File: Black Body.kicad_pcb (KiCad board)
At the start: 2 copper layers, 55 x 53.8 mm, 36 parts, among them IC2 MCP96L00T-E_MX, J1 53307-2471, J3 Conn_01x04, J4 MX150_02x08_RightAngle

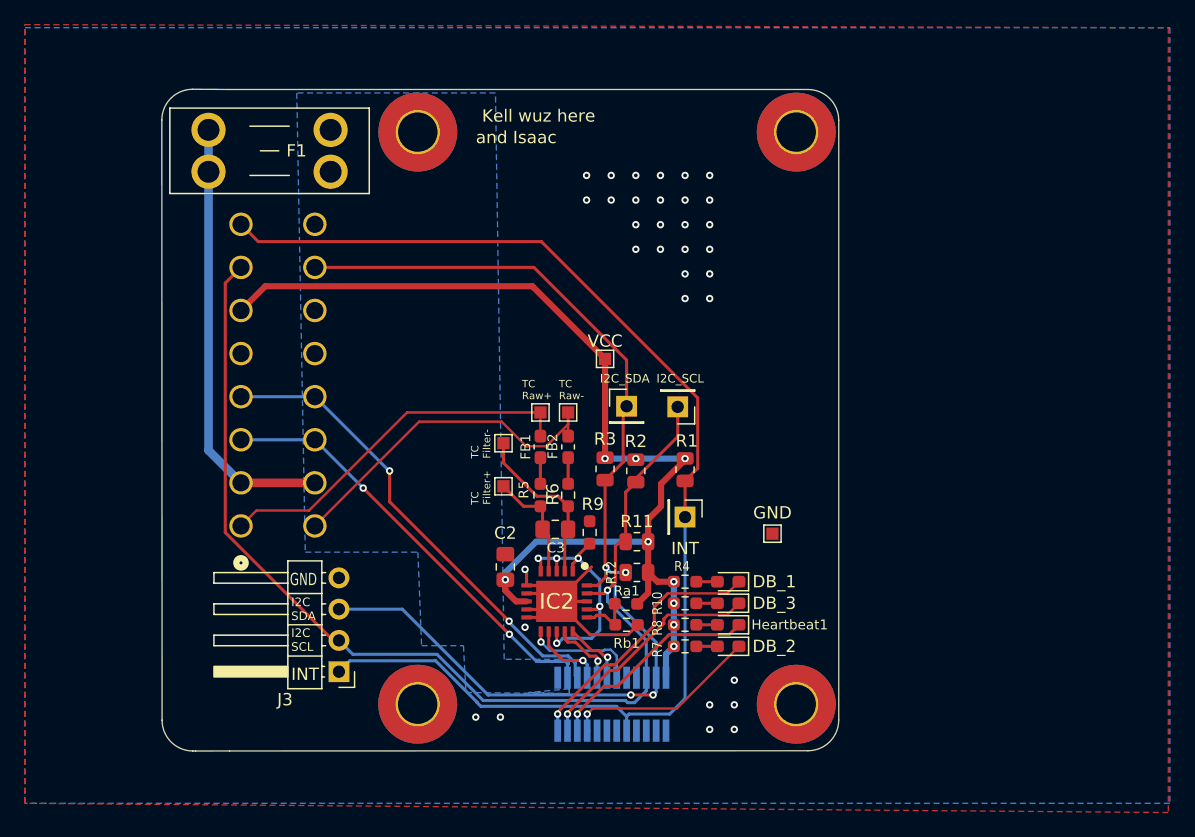
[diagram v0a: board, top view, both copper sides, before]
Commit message: better file system
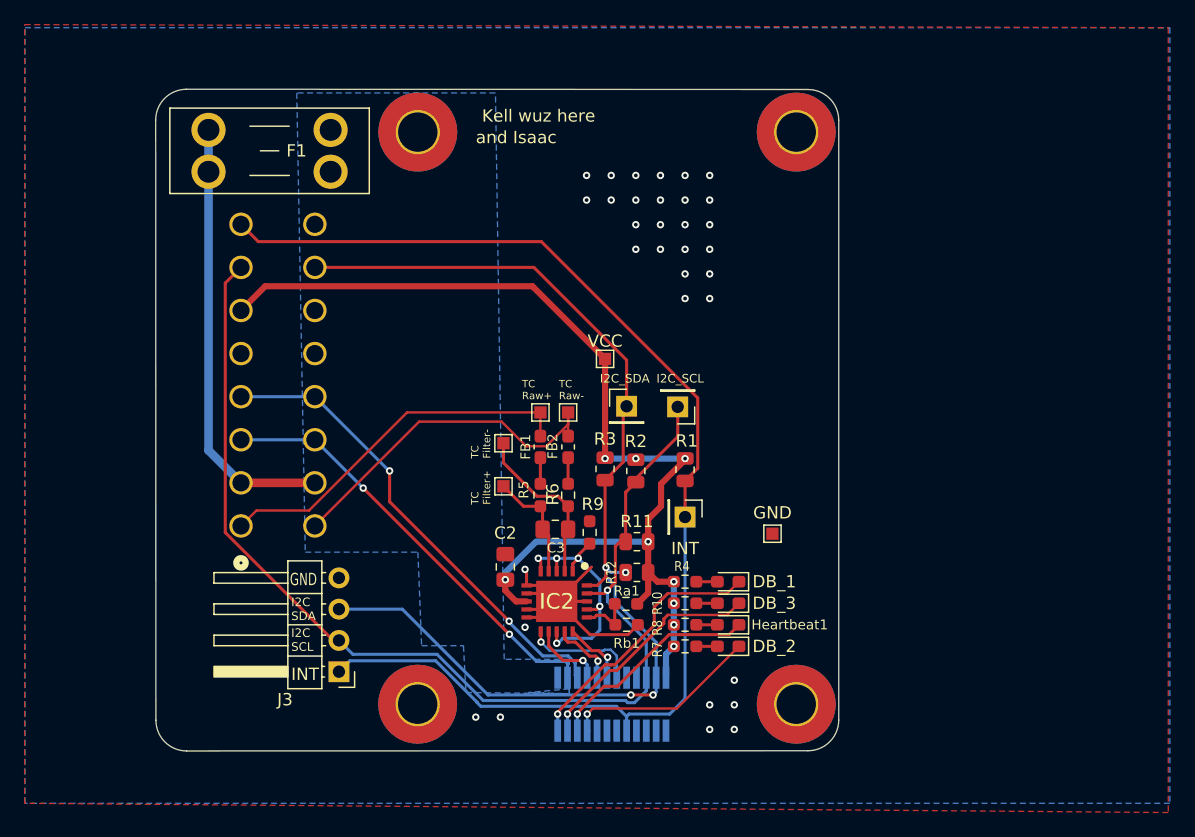
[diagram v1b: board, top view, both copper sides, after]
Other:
- board size 55 x 53.8 mm -> 55.5 x 53.8 mm
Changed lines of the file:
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@@
 		(at 111.05 116.95)
 		(property "Reference" "J1"
-			(at 6.8 -0.67 270)
+			(at 6.8 -0.67 90)
 			(layer "B.SilkS")
 			(effects
@@
 		)
 		(property "Value" "53307-2471"
-			(at 6.5278 5.08 180)
+			(at 6.5278 5.08 0)
 			(layer "B.Fab")
 			(effects
@@
 		)
 		(property "Datasheet" "https://www.molex.com/en-us/products/part-detail-pdf/533072471?display=pdf"
-			(at 0 0 180)
+			(at 0 0 0)
 			(layer "B.Fab")
 			(hide yes)
@@
 		)
 		(property "Description" "Board-to-board connector for Peripheral SOM daughterboards"
-			(at 0 0 180)
+			(at 0 0 0)
 			(layer "B.Fab")
 			(hide yes)
@@
 		)
 		(fp_text user "533072471"
-			(at -5.1816 6.35 180)
+			(at -5.1816 6.35 0)
 			(layer "B.Fab")
 			(effects
@@
 		)
 	)
-	(gr_line
-		(start 77 67)
-		(end 80 67.017767)
-		(stroke
-			(width 0.05)
-			(type default)
-		)
-		(layer "Edge.Cuts")
-	)
 	(gr_arc
 		(start 129.482233 118.232233)
@@
 		(layer "Edge.Cuts")
 	)
-	(gr_line
-		(start 77.25 120.75104)
-		(end 77.017767 120.751128)
-		(stroke
-			(width 0.05)
-			(type default)
-		)
-		(layer "Edge.Cuts")
-	)
-	(gr_line
-		(start 80 120.75)
-		(end 126.982233 120.732233)
-		(stroke
-			(width 0.05)
-			(type default)
-		)
-		(layer "Edge.Cuts")
-	)
 	(gr_arc
 		(start 126.982254 67.017755)
@@
 		(layer "Edge.Cuts")
 	)
-	(gr_line
-		(start 74.5 69.5)
-		(end 74.517767 118.25)
+	(gr_arc
+		(start 74 69.5)
+		(mid 74.732233 67.732233)
+		(end 76.5 67)
 		(stroke
 			(width 0.05)
@@
 		(layer "Edge.Cuts")
 	)
-	(gr_arc
-		(start 74.5 69.5)
-		(mid 75.232233 67.732233)
-		(end 77 67)
+	(gr_line
+		(start 129.482233 118.232233)
+		(end 129.482254 69.517755)
 		(stroke
 			(width 0.05)
@@
 	)
 	(gr_line
-		(start 129.482233 118.232233)
-		(end 129.482254 69.517755)
+		(start 126.9822 67.017755)
+		(end 76.5 67)
 		(stroke
 			(width 0.05)
@@
 	)
 	(gr_line
-		(start 80 67.017767)
-		(end 126.982254 67.017755)
+		(start 76.51779 120.75)
+		(end 126.982233 120.732233)
 		(stroke
 			(width 0.05)
@@
 		(layer "Edge.Cuts")
 	)
-	(gr_arc
-		(start 77.017767 120.75)
-		(mid 75.25 120.017767)
-		(end 74.517767 118.25)
+	(gr_line
+		(start 74 69.5)
+		(end 74.017767 118.25)
 		(stroke
 			(width 0.05)
@@
 		(layer "Edge.Cuts")
 	)
-	(gr_line
-		(start 80 120.75)
-		(end 77.25 120.75104)
+	(gr_arc
+		(start 76.517767 120.75)
+		(mid 74.75 120.017767)
+		(end 74.017767 118.25)
 		(stroke
 			(width 0.05)
@@
 			)
 		)
+	)
+	(zone
+		(net 37)
+		(net_name "/INT")
+		(layer "B.Cu")
+		(name "$teardrop_padvia$")
+		(hatch none 0.1)
+		(priority 30000)
+		(attr
+			(teardrop
+				(type padvia)
+			)
+		)
+		(connect_pads yes
+			(clearance 0)
+		)
+		(min_thickness 0.0254)
+		(filled_areas_thickness no)
+		(fill yes
+			(thermal_gap 0.5)
+			(thermal_bridge_width 0.5)
+			(island_removal_mode 1)
+			(island_area_min 10)
+		)
+		(polygon
+			(pts
+				(xy 98.368253 114.874958) (xy 98.191476 115.051735) (xy 97.611064 114.219905) (xy 96.070707 116.950707)
+				(xy 98.948666 115.706789)
+			)
+		)
